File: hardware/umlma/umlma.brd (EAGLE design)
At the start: 17.7 x 16.8 mm, 13 parts, among them IC1 TINY25, J1 AVRISP6_TP

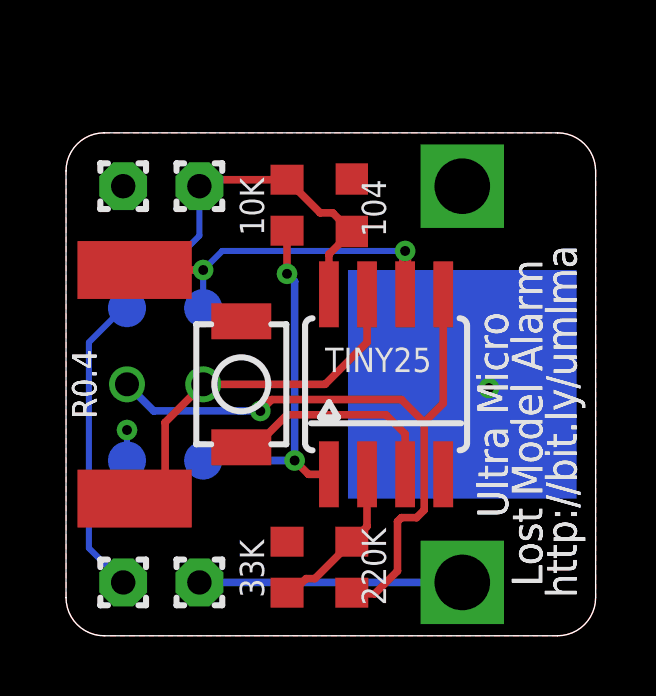
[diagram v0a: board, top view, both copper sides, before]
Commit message: updated layout, silk, gerbers, zip
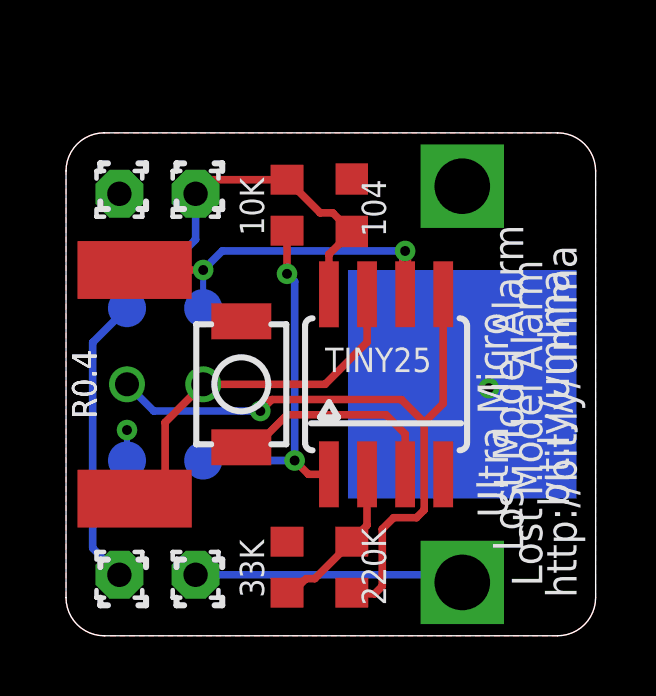
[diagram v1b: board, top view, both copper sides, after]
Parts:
- added U$1: BTLOGO-LOGO-SM, bt:BTLOGOS
- moved PAD4 0.28 mm to (4.32, 14.7)
- moved PAD3 0.28 mm to (1.78, 14.7)
- moved PAD2 0.28 mm to (4.32, 2.03)
- moved PAD1 0.28 mm to (1.78, 2.03)
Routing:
- net VCC: track 23.6 -> 23.0 mm
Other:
- board text added: "bit.ly/umlma"
